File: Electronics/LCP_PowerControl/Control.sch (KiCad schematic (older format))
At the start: 2 parts, among them J2 Conn_01x05_Shielded

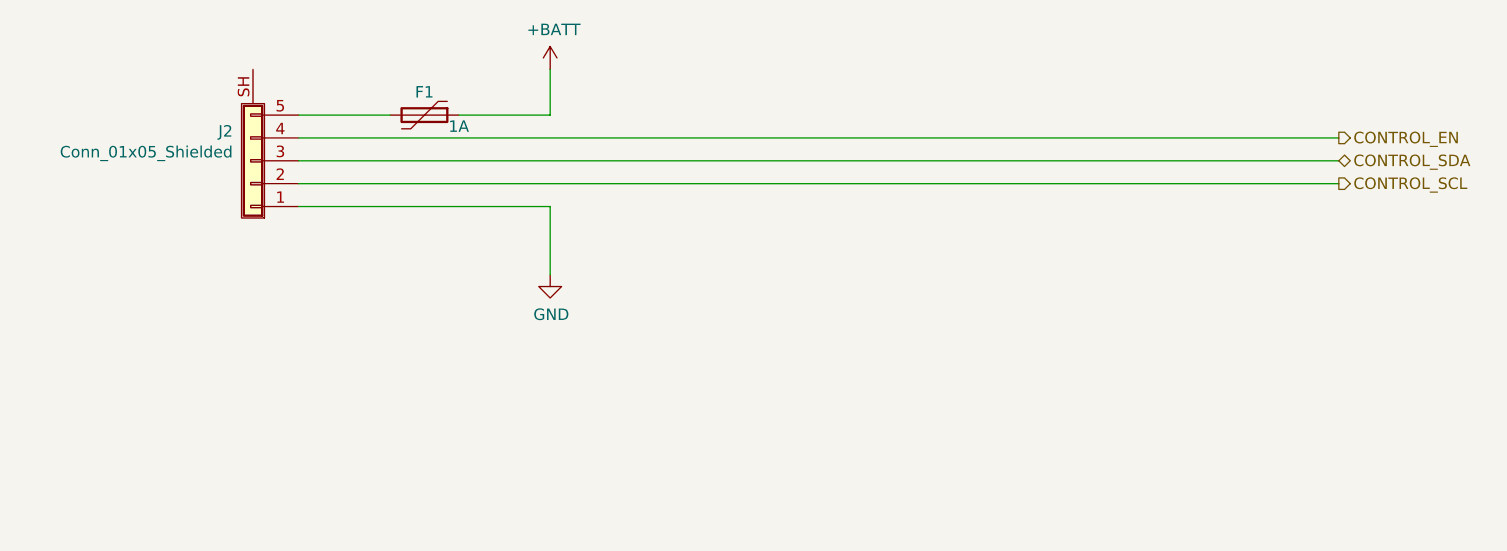
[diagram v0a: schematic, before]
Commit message: Adding libraries and recent changes
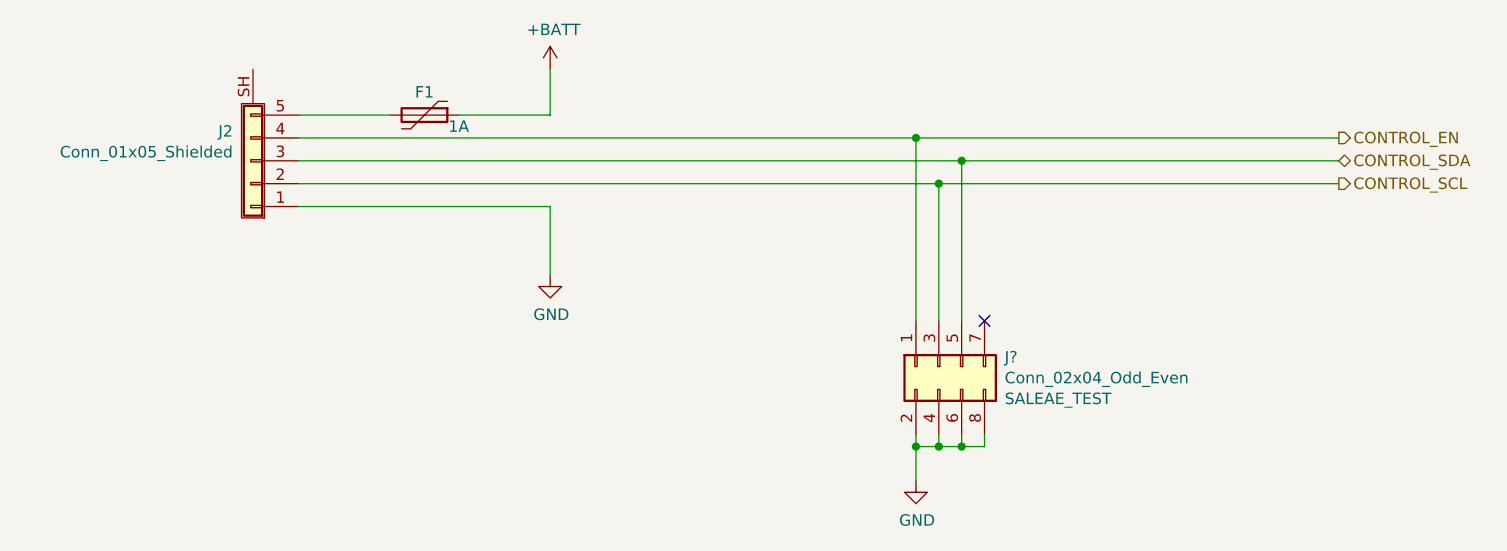
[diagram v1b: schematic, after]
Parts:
- added J?: Conn_02x04_Odd_Even, Connector_PinSocket_2.54mm:PinSocket_2x04_P2.54mm_Vertical, symbol Connector_Generic:Conn_02x04_Odd_Even
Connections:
- net CONTROL_EN: now also J?.1 (Pin_1)
- net CONTROL_SCL: now also J?.3 (Pin_3)
- net CONTROL_SDA: now also J?.5 (Pin_5)
- net GND: now also J?.2 (Pin_2), J?.4 (Pin_4), J?.6 (Pin_6), J?.8 (Pin_8)
- no-connect marks 0 -> 1
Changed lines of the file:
@@
 $Descr A4 11693 8268
 encoding utf-8
-Sheet 6 8
+Sheet 5 11
 Title ""
 Date ""
@@
 CONTROL_SCL
 Wire Wire Line
-	8950 3700 4400 3700
+	8950 3800 7300 3800
 Wire Wire Line
-	8950 3800 4400 3800
-Wire Wire Line
-	4400 3900 8950 3900
+	4400 3900 7200 3900
 $Comp
 L power:GND #PWR010
@@
 Wire Wire Line
 	4400 3600 4800 3600
+$Comp
+L power:GND #PWR?
+U 1 1 5EED44A2
+P 7100 5200
+F 0 "#PWR?" H 7100 4950 50  0001 C CNN
+F 1 "GND" H 7105 5027 50  0000 C CNN
+F 2 "" H 7100 5200 50  0001 C CNN
+F 3 "" H 7100 5200 50  0001 C CNN
+	1    7100 5200
+	1    0    0    -1
+$EndComp
+Wire Wire Line
+	7100 5200 7100 5050
+Wire Wire Line
+	7200 5000 7200 5050
+Wire Wire Line
+	7200 5050 7100 5050
+Connection ~ 7100 5050
+Wire Wire Line
+	7100 5050 7100 5000
+Wire Wire Line
+	7300 5000 7300 5050
+Connection ~ 7200 5050
+$Comp
+L Connector_Generic:Conn_02x04_Odd_Even J?
+U 1 1 5EED0364
+P 7200 4700
+F 0 "J?" V 7159 4412 50  0000 R CNN
+F 1 "Conn_02x04_Odd_Even" V 7250 4412 50  0000 R CNN
+F 2 "Connector_PinSocket_2.54mm:PinSocket_2x04_P2.54mm_Vertical" H 7200 4700 50  0001 C CNN
+F 3 "~" H 7200 4700 50  0001 C CNN
+F 4 "SALEAE_TEST" V 7341 4412 50  0000 R CNN "Field4"
+	1    7200 4700
+	0    -1   1    0
+$EndComp
+Wire Wire Line
+	7400 5000 7400 5050
+Wire Wire Line
+	7200 5050 7300 5050
+Wire Wire Line
+	7300 5050 7400 5050
+Connection ~ 7300 5050
+Wire Wire Line
+	7100 4500 7100 3700
+Wire Wire Line
+	4400 3700 7100 3700
+Connection ~ 7100 3700
+Wire Wire Line
+	7100 3700 8950 3700
+Wire Wire Line
+	7200 4500 7200 3900
+Connection ~ 7200 3900
+Wire Wire Line
+	7200 3900 8950 3900
+Wire Wire Line
+	7300 4500 7300 3800
+Connection ~ 7300 3800
+Wire Wire Line
+	7300 3800 4400 3800
+NoConn ~ 7400 4500
 $EndSCHEMATC
